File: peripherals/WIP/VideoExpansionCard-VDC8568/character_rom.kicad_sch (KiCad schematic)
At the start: 2 parts, among them U6 74HCT273, U8 27C64

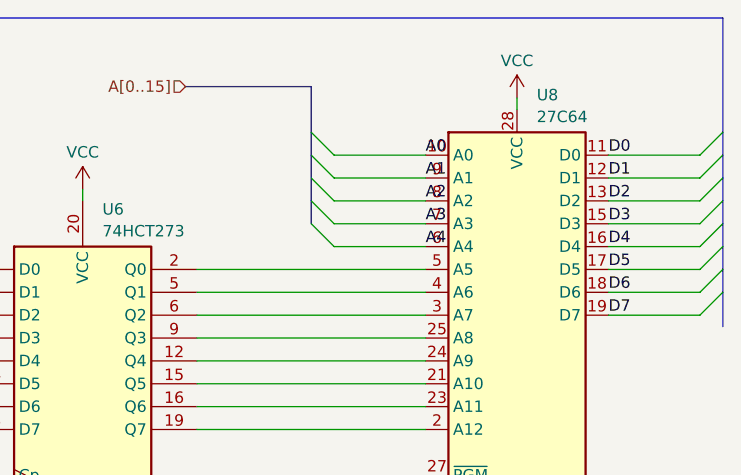
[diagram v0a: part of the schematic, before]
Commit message: Updates to a lot!
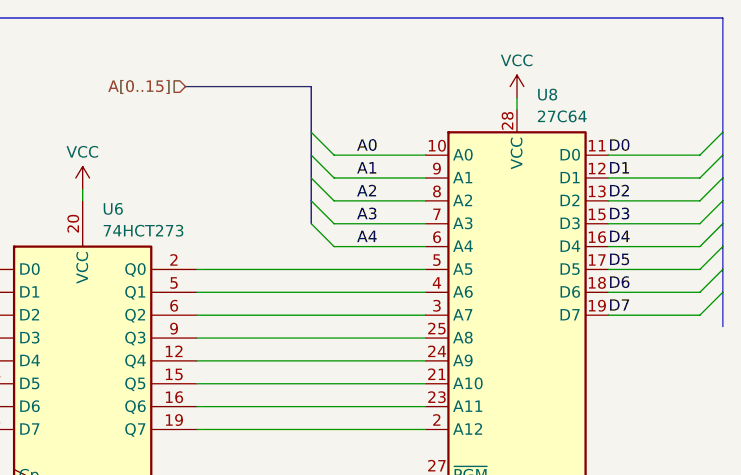
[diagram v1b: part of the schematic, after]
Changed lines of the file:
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@@
 	)
 	(label "A1"
-		(at 148.59 35.56 0)
+		(at 140.97 35.56 0)
 		(fields_autoplaced yes)
 		(effects
@@
 	)
 	(label "A0"
-		(at 148.59 33.02 0)
+		(at 140.97 33.02 0)
 		(fields_autoplaced yes)
 		(effects
@@
 	)
 	(label "A4"
-		(at 148.59 43.18 0)
+		(at 140.97 43.18 0)
 		(fields_autoplaced yes)
 		(effects
@@
 	)
 	(label "A2"
-		(at 148.59 38.1 0)
+		(at 140.97 38.1 0)
 		(fields_autoplaced yes)
 		(effects
@@
 	)
 	(label "A3"
-		(at 148.59 40.64 0)
+		(at 140.97 40.64 0)
 		(fields_autoplaced yes)
 		(effects
